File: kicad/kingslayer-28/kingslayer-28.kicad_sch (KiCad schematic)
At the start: 75 parts, among them IC1 STM32F303CCT7, IC3 LM3940IMP-3.3_NOPB, K1 KEYSW, K10 KEYSW, K11 KEYSW, K12 KEYSW, K13 KEYSW, K14 KEYSW, K15 KEYSW, K16 KEYSW, K17 KEYSW, K18 KEYSW, K19 KEYSW, K2 KEYSW, K20 KEYSW, K21 KEYSW, K22 KEYSW, K23 KEYSW, K24 KEYSW, K25 KEYSW, K26 KEYSW, K27 KEYSW, K28 KEYSW, K3 KEYSW, K4 KEYSW, K5 KEYSW, K6 KEYSW, K7 KEYSW, K8 KEYSW, K9 KEYSW, SW1 MSS13PLP, X1 IC21008.000M30.0EE1B

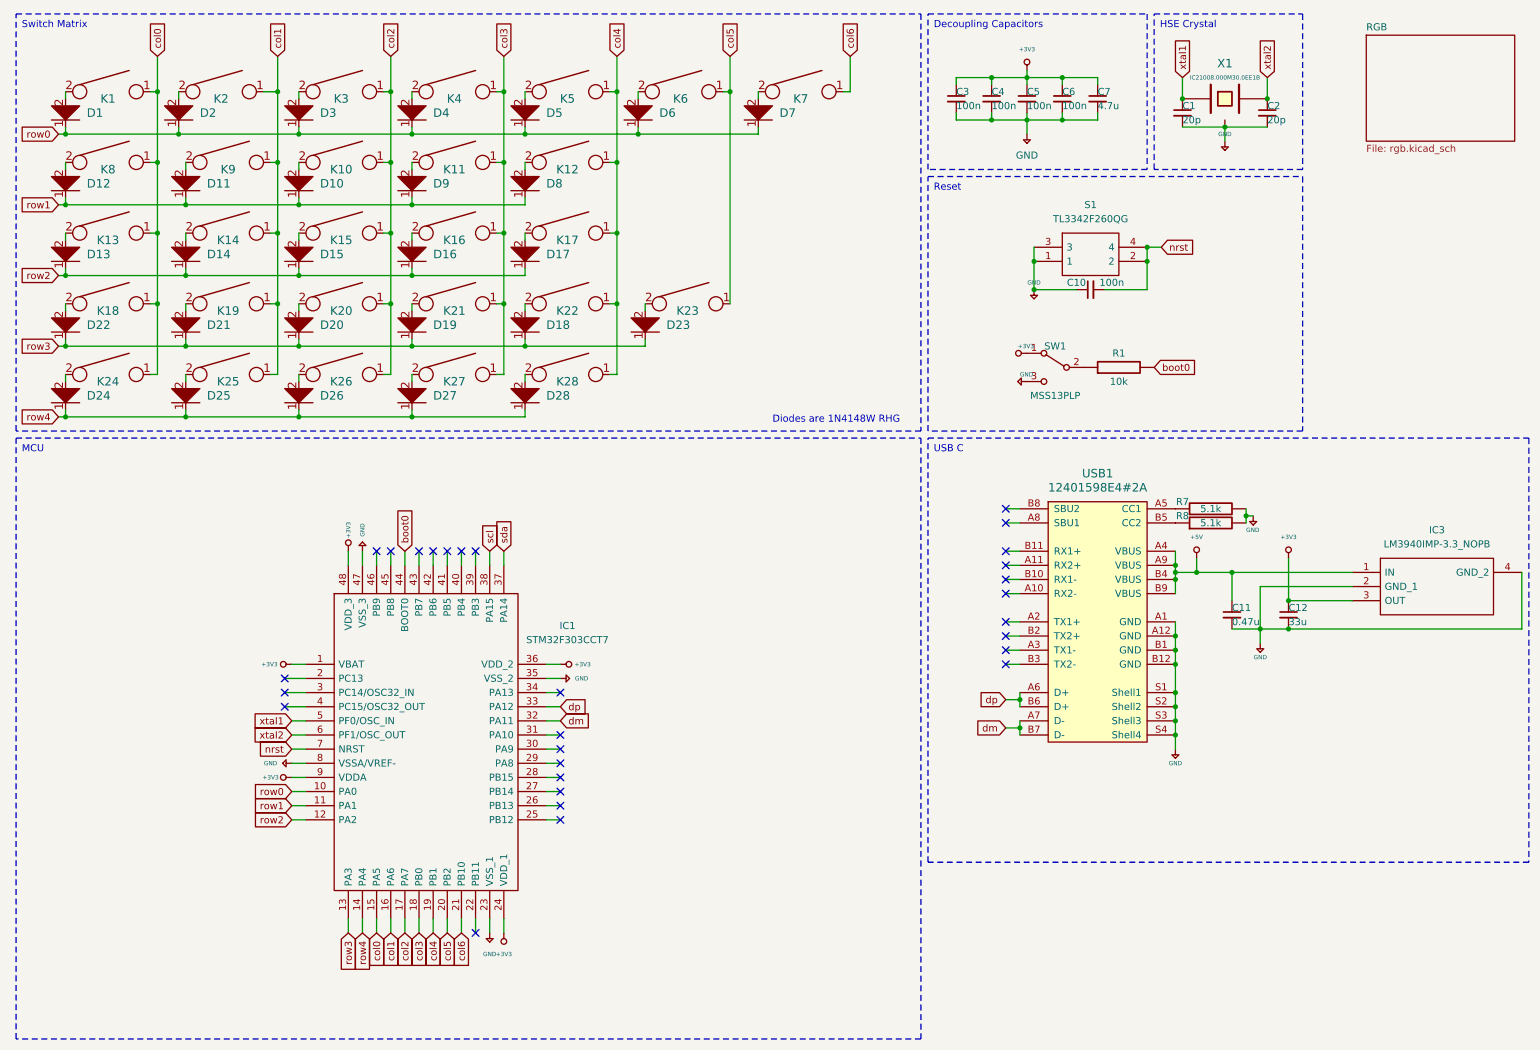
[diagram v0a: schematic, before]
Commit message: Addressed some comments
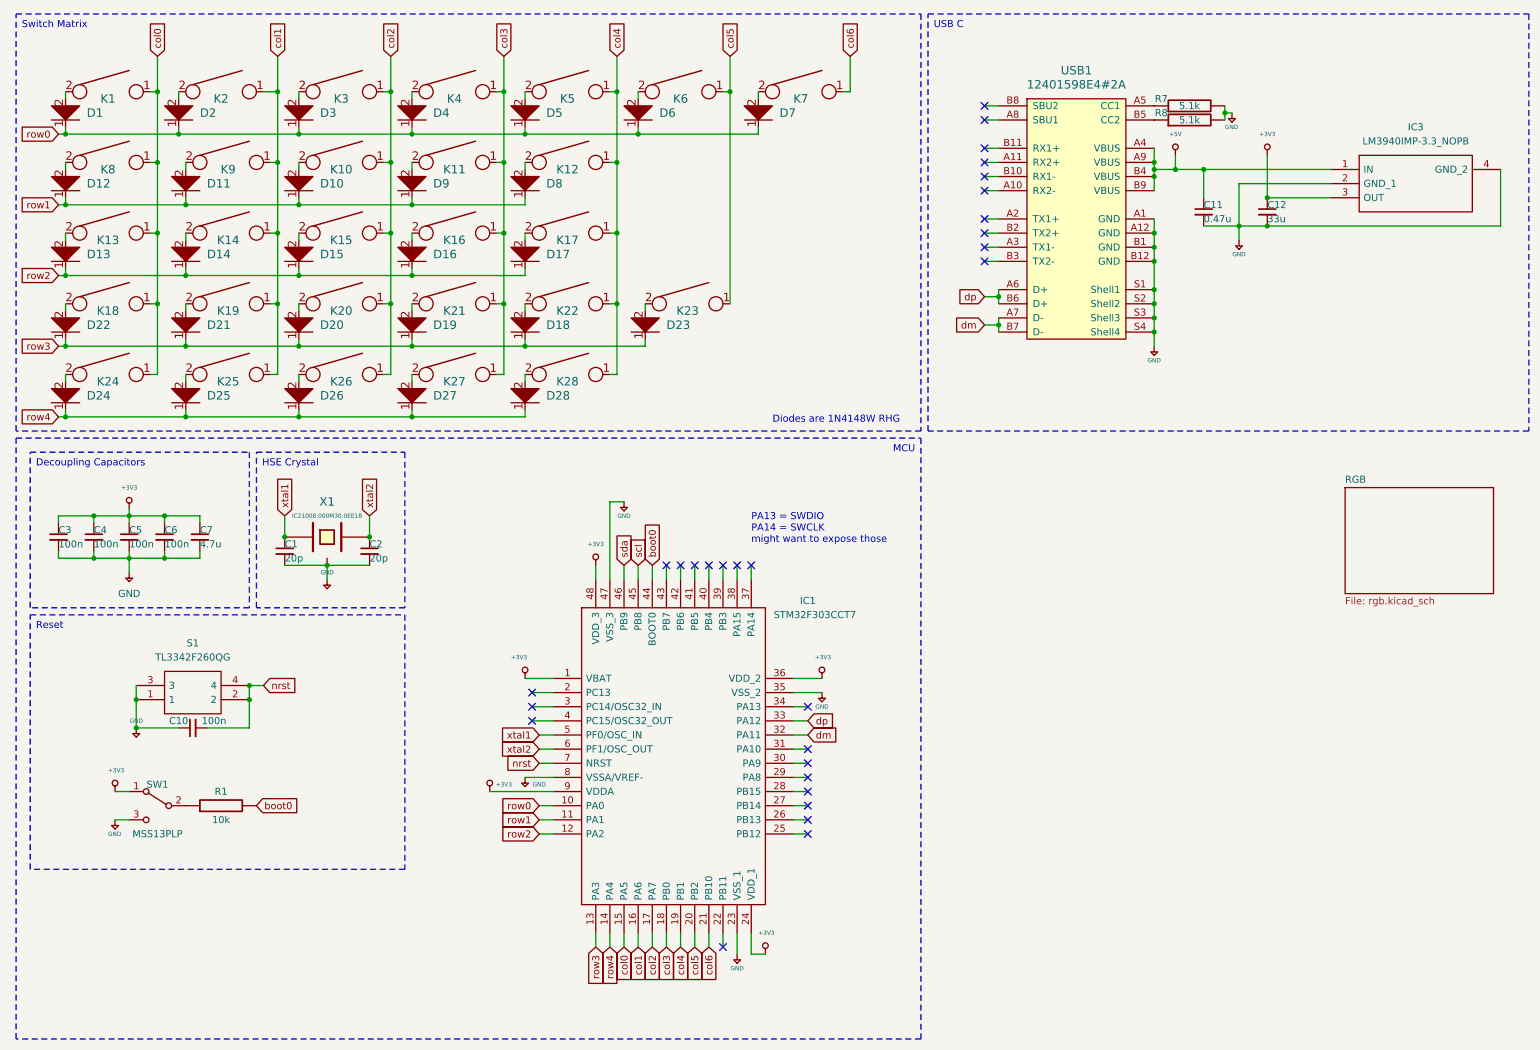
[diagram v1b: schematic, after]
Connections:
- net scl: now also IC1.45 (PB8); no longer IC1.38 (PA15)
- net sda: now also IC1.46 (PB9); no longer IC1.37 (PA14)
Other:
- note added: "PA13 = SWDIO PA14 = SWCLK might want to expose those"
- moved on the sheet: C1, C10, C11, C12, C2, C3, C4, C5, C6, C7, IC1, IC3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
